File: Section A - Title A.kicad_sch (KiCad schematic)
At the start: 40 parts, among them U1 AD7190WBRUZ, Y1 ABC2-4.9152MHZ-4-T

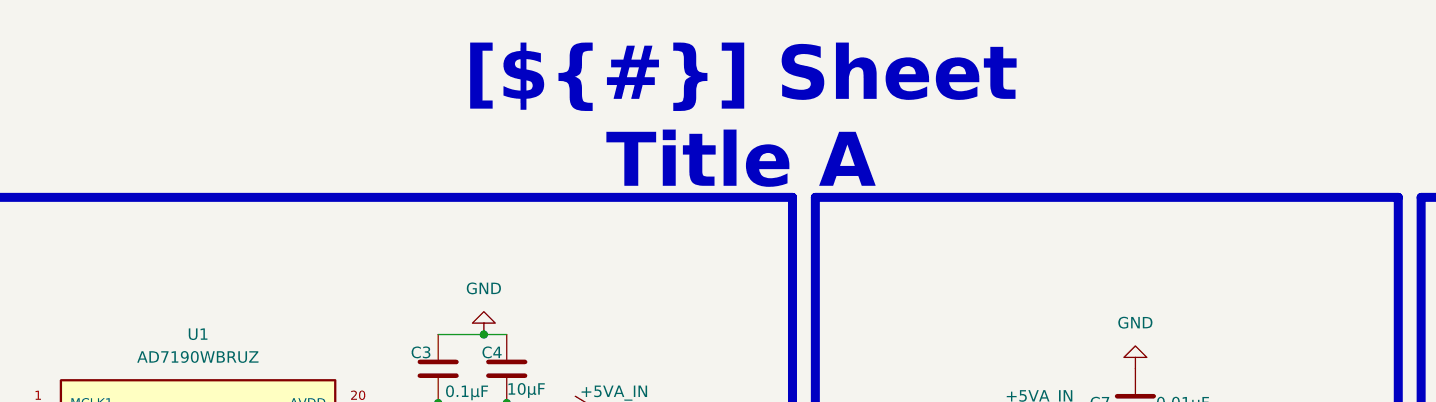
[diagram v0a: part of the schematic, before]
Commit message: [Finish schématiq]
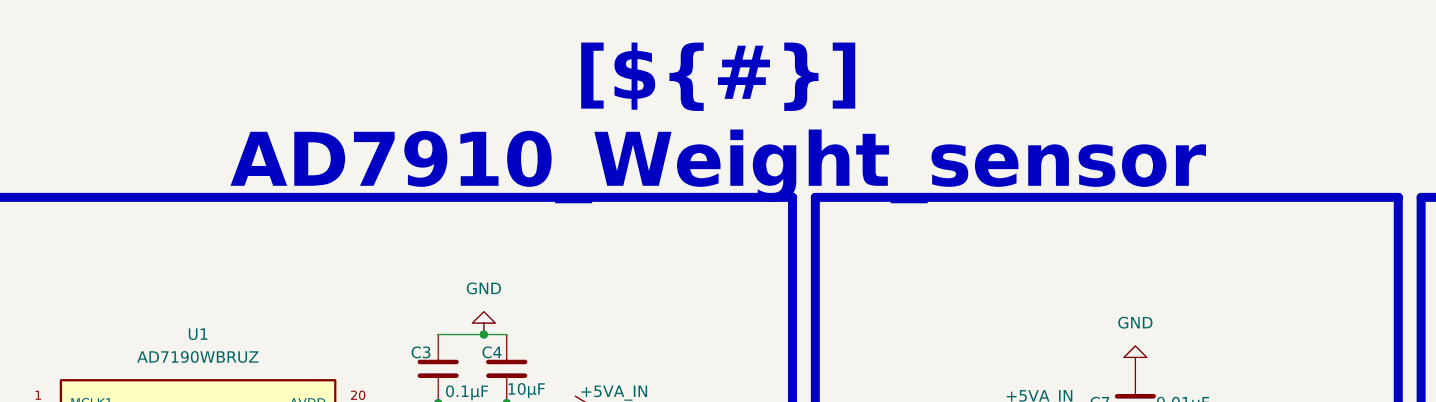
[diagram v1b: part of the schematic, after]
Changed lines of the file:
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@@
 		)
 	)
-	(text_box "[${#}] ${TITLE}"
+	(text_box "[${#}] AD7910_Weight_sensor"
 		(exclude_from_sim no)
-		(at 115.57 15.24 0)
-		(size 72.39 12.7)
+		(at 92.71 15.24 0)
+		(size 113.03 12.7)
 		(margins 4.4999 4.4999 4.4999 4.4999)
 		(stroke
 			(width -0.0001)
-			(type default)
+			(type solid)
 		)
 		(fill
